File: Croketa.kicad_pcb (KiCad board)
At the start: 2 copper layers, 17.8 x 33 mm, 24 parts, among them J1 USB_B_Micro, J2 Conn_02x02_Odd_Even, P1 Digital, P4 Analog, SW1 SW_DPST_x2, U1 AP2112K-3.3TRG1, U2 ATSAMD21E18A-AF

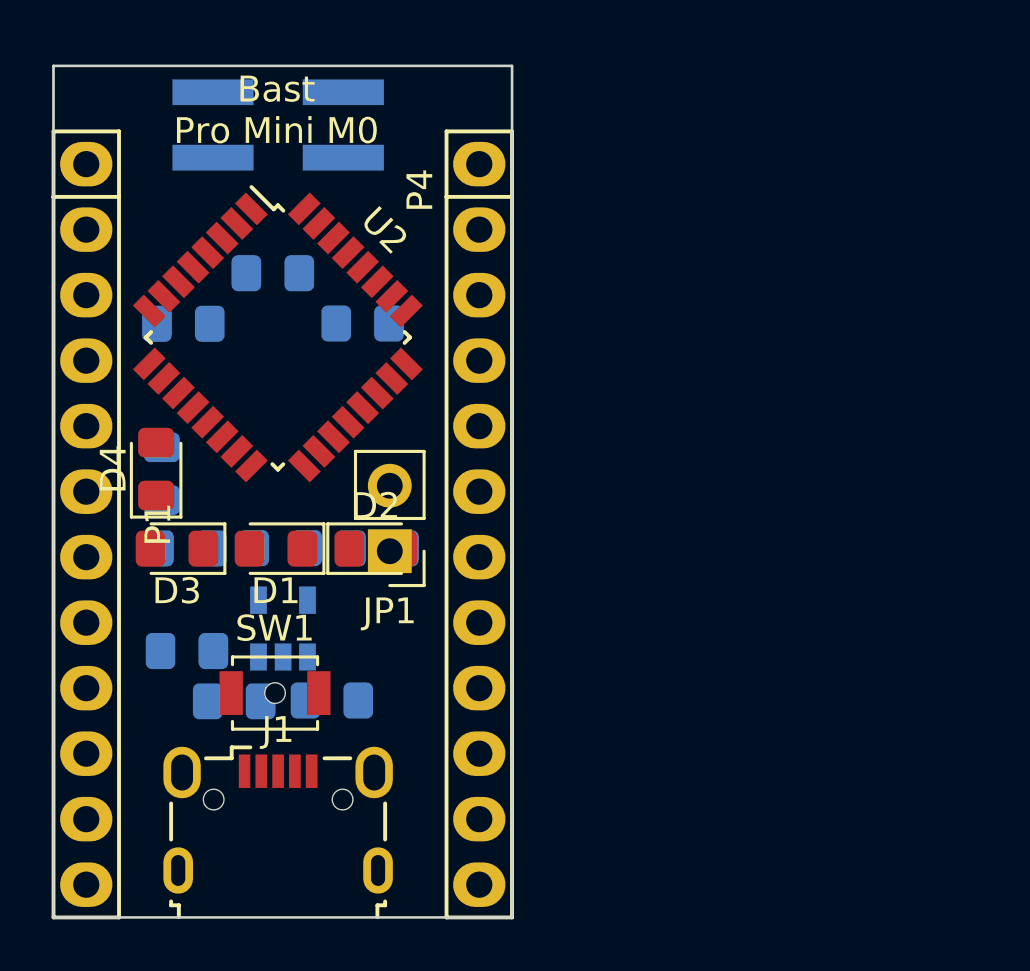
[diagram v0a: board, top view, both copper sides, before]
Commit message: Pre router
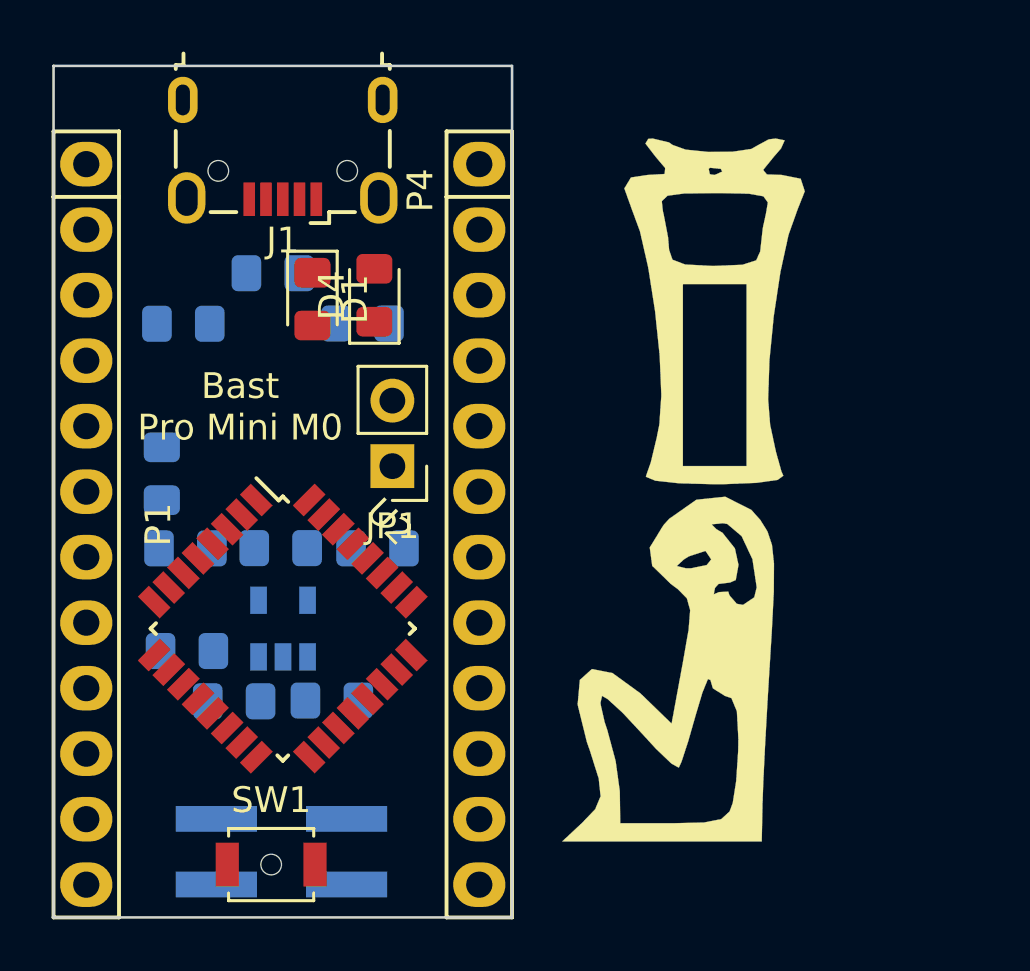
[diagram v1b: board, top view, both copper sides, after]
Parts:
- removed D2, D3: LED, LED_SMD:LED_0805_2012Metric_Pad1.15x1.40mm_HandSolder
- added G***: LOGO, LOGO, F.Cu at (160.9, 104.7)
- added G***: LOGO, LOGO, F.Cu at (162.8, 90.8)
- moved J2 28.2 mm to (146.0, 111.8)
- moved J1 26.0 mm to (146.1, 84.5), turned to 180 degrees
- moved U2 11.3 mm to (146.1, 103.1)
- moved D4 10.8 mm to (149.6, 90.2)
- moved D1 9.78 mm to (147.2, 90.3), turned to 270 degrees
- moved SW1 6.65 mm to (145.6, 112.2)
- moved JP1 3.30 mm to (150.3, 96.8)

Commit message: Dimensions of Bast Pro Mini M0
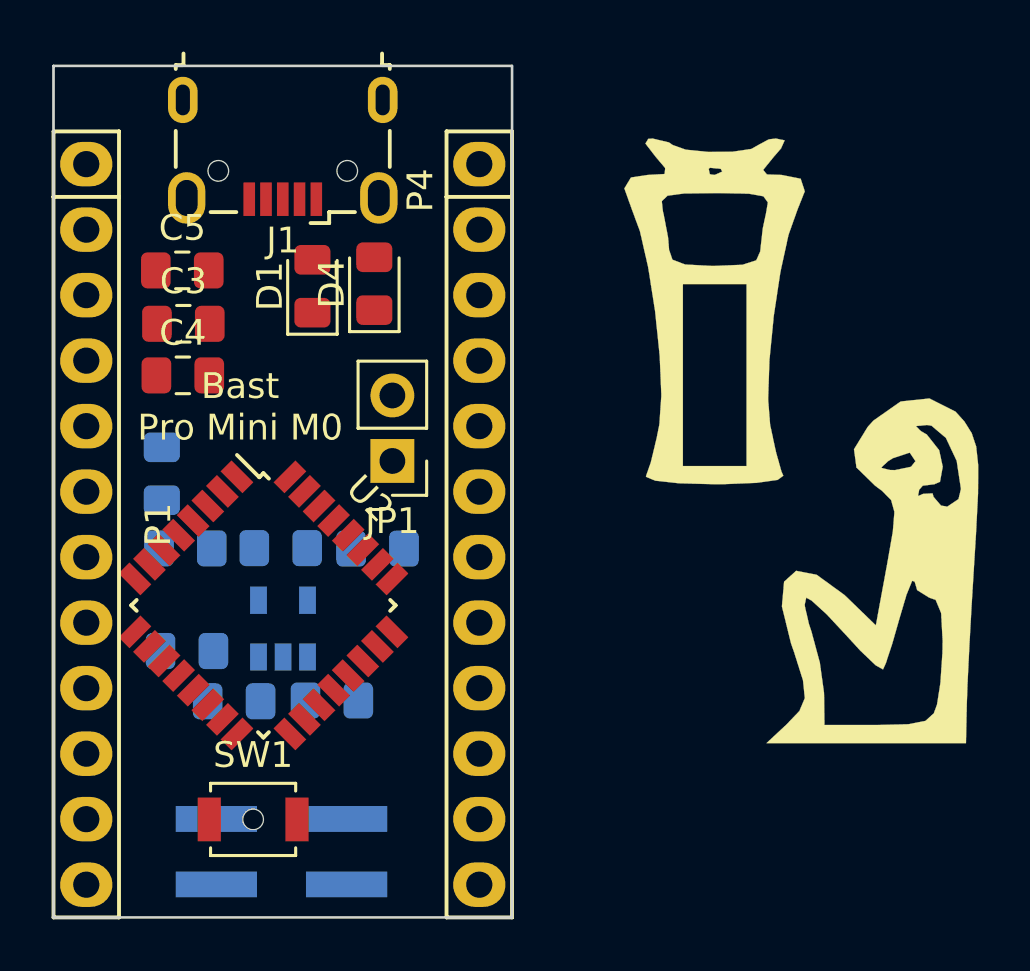
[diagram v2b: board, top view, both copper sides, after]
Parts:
- C3, C4, C5: moved to F.Cu
- D1: value LED -> POWER
- moved G*** 8.79 mm to (168.8, 100.8)
- moved C4 7.25 mm to (142.2, 93.3)
- moved C5 3.51 mm to (142.2, 89.2), turned to 0 degrees
- moved SW1 1.88 mm to (144.9, 110.5)
- moved U2 1.17 mm to (145.3, 102.2)
- moved D1 0.50 mm to (147.2, 89.8), turned to 90 degrees
- moved D4 0.45 mm to (149.6, 89.7)
- moved JP1 0.20 mm to (150.3, 96.6)
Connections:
- net /AREF renamed Net-(U2-Pad4)
- C1 pad 1: +5V -> VCC
- F1 pad 1: +5V -> VCC
- J1 pad 2: Net-(J1-Pad2) -> /D-
- J1 pad 3: Net-(J1-Pad3) -> /D+
- P1 pad 3: /Reset -> /RESET
- R2 pad 2: /TX_LED -> /LED
- SW1 pad 1: /Reset -> /RESET
- U1 pad 1: +5V -> VCC
- U1 pad 3: +5V -> VCC
- U2 pad 11: /4 -> /SDA
- U2 pad 12: /3(**) -> /SCL
- U2 pad 14: /A4 -> /LED
- U2 pad 21: /SDA -> /4
- U2 pad 22: /SCL -> /3(**)
- U2 pad 23: /USB_D- -> /D-
- U2 pad 24: /USB_D+ -> /D+
- U2 pad 25: /TX_LED -> /6(**)
- U2 pad 27: /USB_HOST_EN -> /7
